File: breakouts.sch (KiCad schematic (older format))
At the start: 8 parts

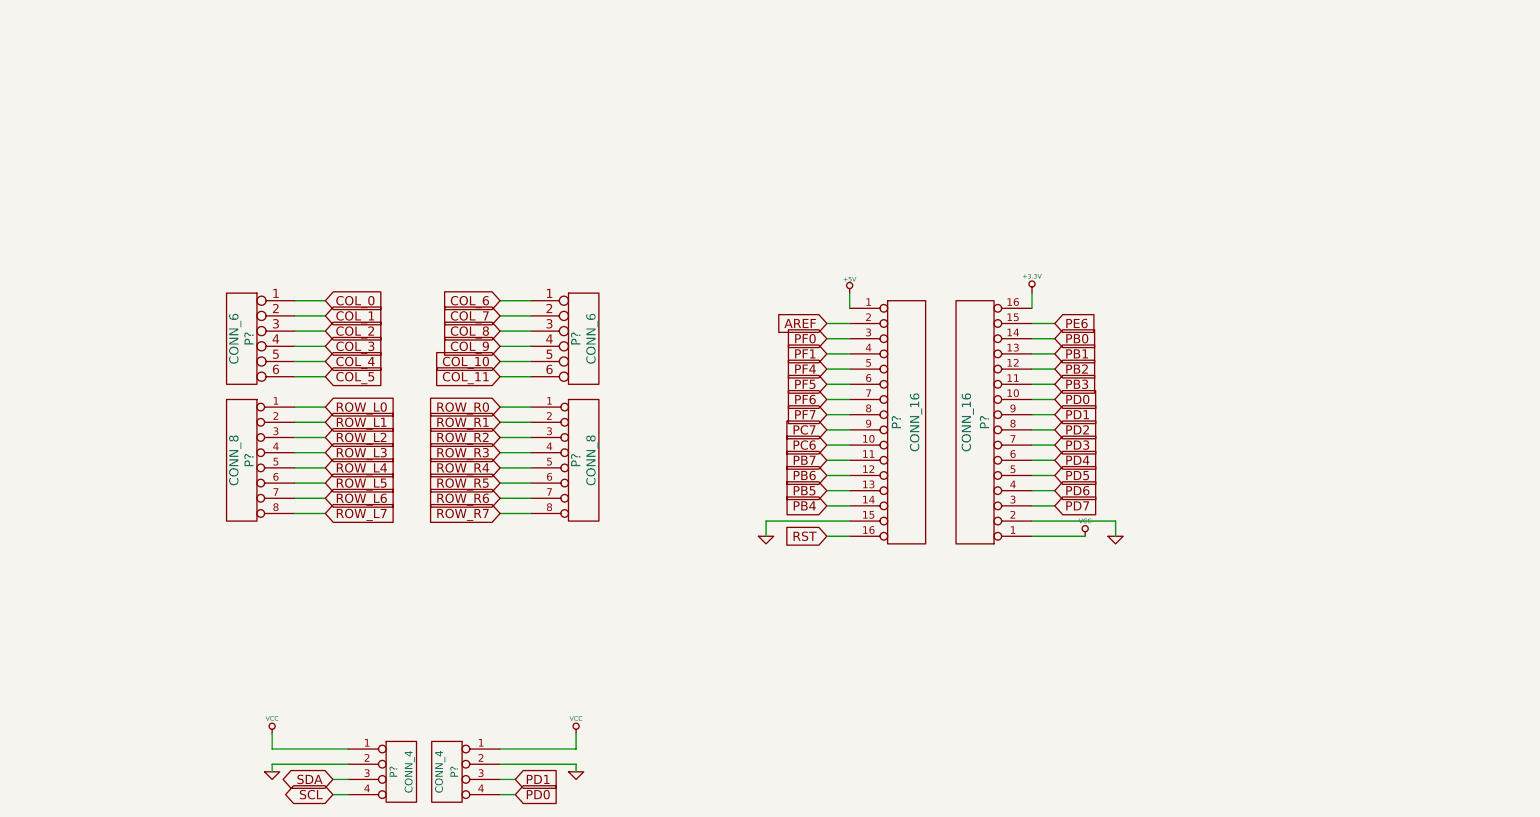
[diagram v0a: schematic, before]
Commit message: Sort remaining sections to sheets
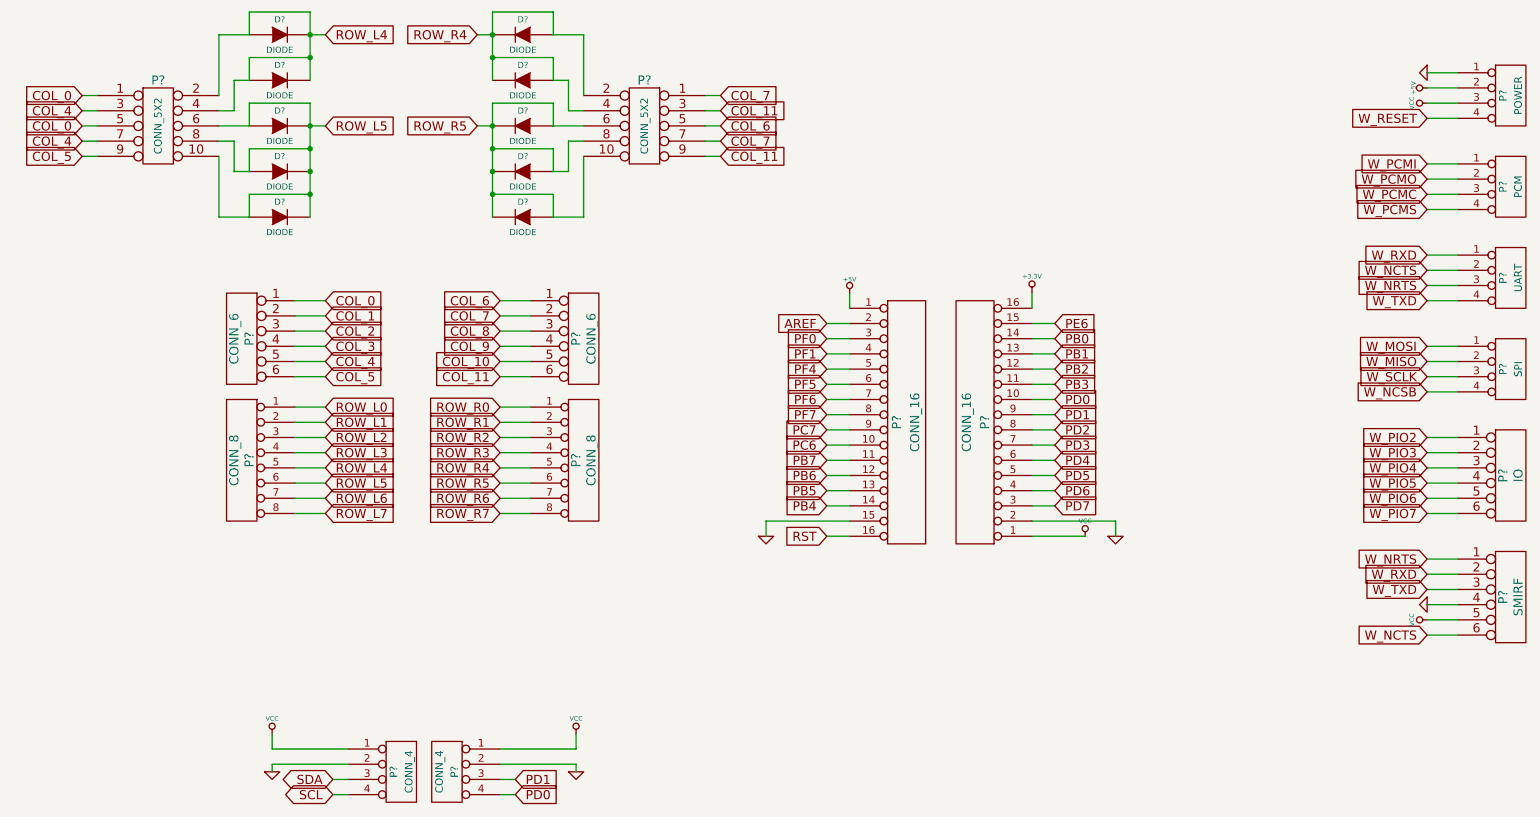
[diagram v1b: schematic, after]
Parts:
- added D? (x10): DIODE, symbol DIODE
- added P?: SMIRF, symbol CONN_6
- added P?: IO, symbol CONN_6
- added P?: SPI, symbol CONN_4
- added P?: UART, symbol CONN_4
- added P?: PCM, symbol CONN_4
- added P?: POWER, symbol CONN_4
- added P? (x2): CONN_5X2, symbol CONN_5X2
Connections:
- net +5V: now also P?.2 (P2)
- net COL_0: now also P?.1, P?.5
- net COL_11: now also P?.3, P?.9
- net COL_4: now also P?.3, P?.7
- net COL_5: now also P?.9
- net COL_6: now also P?.5
- net COL_7: now also P?.1, P?.7
- net GND: now also P?.1 (P1), P?.4
- net ROW_L4: now also D?.1 (A), D?.1 (A), D?.2 (K), D?.2 (K), P?.2, P?.4
- net ROW_L5: now also D?.1 (A), D?.1 (A), D?.1 (A), D?.2 (K), D?.2 (K), D?.2 (K), P?.10, P?.6, P?.8
- net ROW_R4: now also D?.1 (A), D?.1 (A), D?.2 (K), D?.2 (K), P?.2, P?.4
- net ROW_R5: now also D?.1 (A), D?.1 (A), D?.1 (A), D?.2 (K), D?.2 (K), D?.2 (K), P?.10, P?.6, P?.8
- net VCC: now also P?.3 (P3), P?.5
- new net W_MISO: P?.2 (P2)
- new net W_MOSI: P?.1 (P1)
- new net W_NCSB: P?.4 (P4)
- new net W_NCTS: P?.2 (P2), P?.6
- new net W_NRTS: P?.1, P?.3 (P3)
- new net W_PCMC: P?.3 (P3)
- new net W_PCMI: P?.1 (P1)
- new net W_PCMO: P?.2 (P2)
- new net W_PCMS: P?.4 (P4)
- new net W_PIO2: P?.1
- new net W_PIO3: P?.2
- new net W_PIO4: P?.3
- new net W_PIO5: P?.4
- new net W_PIO6: P?.5
- new net W_PIO7: P?.6
- new net W_RESET: P?.4 (P4)
- new net W_RXD: P?.1 (P1), P?.2
- new net W_SCLK: P?.3 (P3)
- new net W_TXD: P?.3, P?.4 (P4)
